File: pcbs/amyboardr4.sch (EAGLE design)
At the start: 129 parts, among them J1 52601-G10-8LF, M13 M2.5, M14 M2.5, M15 M2.5, M16 M2.5, Q2 S8050, Q5 S8050, U1 PCM9211PT, U13 HX3608, U15 H11L1SR2M, U16 SPX3819, U2 ESP32­S2­SOLO, Y1 ABM10W-22.5792MHZ-8-K1Z-T3

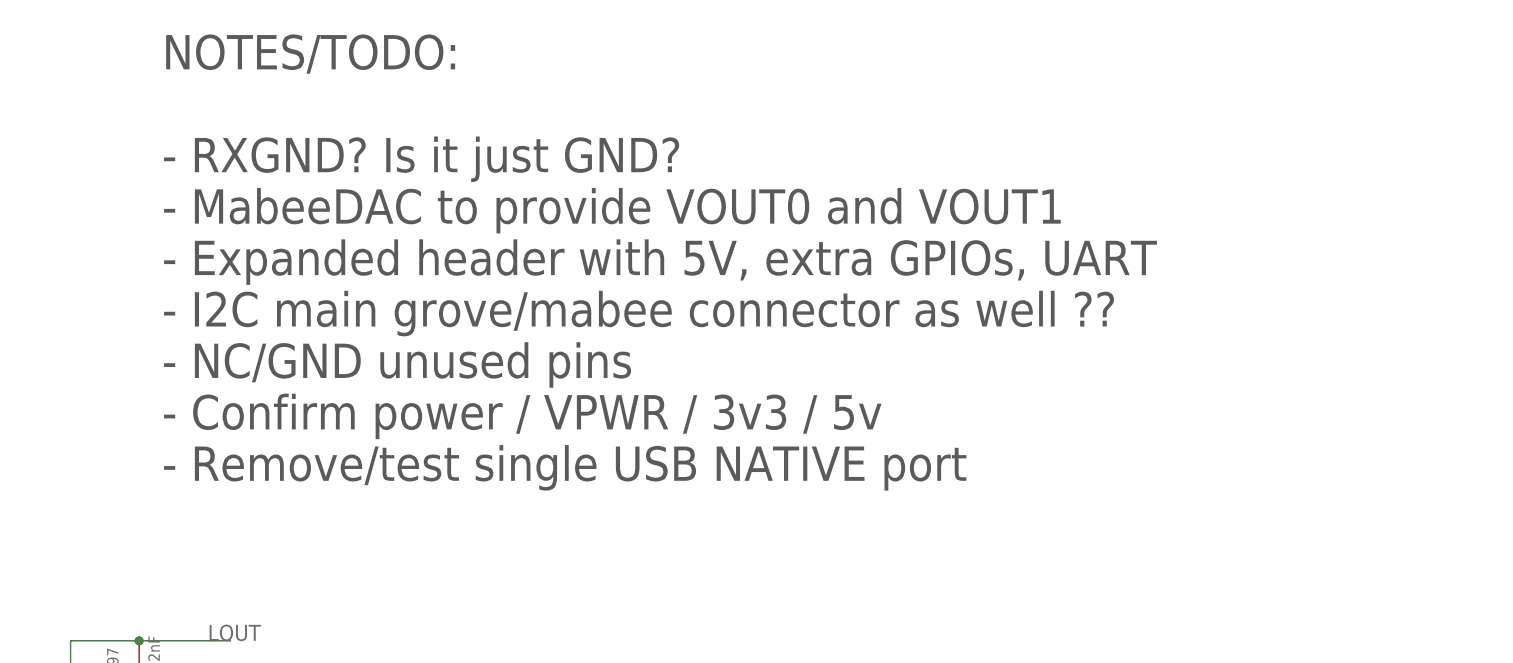
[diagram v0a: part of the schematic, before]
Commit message: .
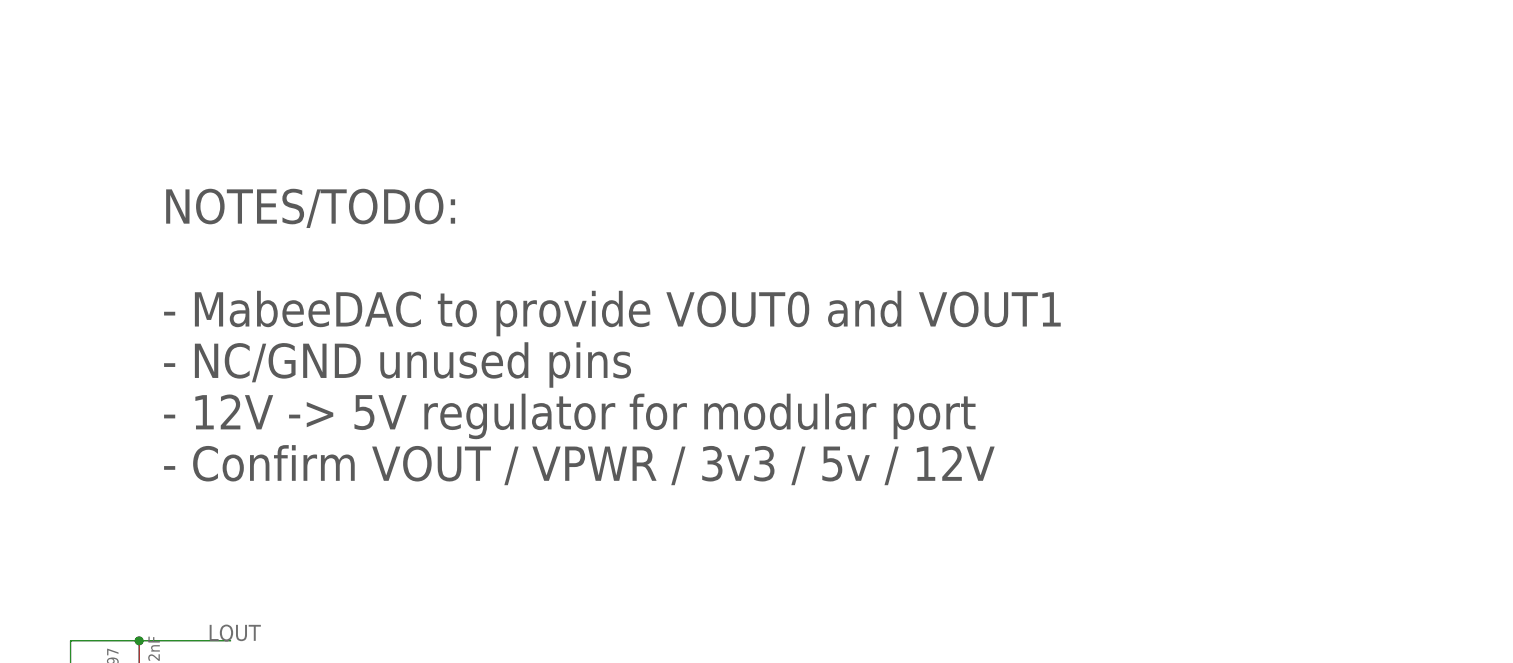
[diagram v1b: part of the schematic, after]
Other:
- note added: "NOTES/TODO: - MabeeDAC to provide VOUT0 and VOUT1 - NC/GND unused pins - 12V -> 5V regulator for modular port - Confirm VOUT / VPWR / 3v3 / 5v / 12V"
- note removed: "NOTES/TODO: - RXGND? Is it just GND? - MabeeDAC to provide VOUT0 and VOUT1 - Expanded header with 5V, extra GPIOs, UART - I2C main grove/mabee connector as well ?? - NC/GND unused pins - Confirm power / VPWR / 3v3 / 5v - Remove/test single USB NATIVE port"
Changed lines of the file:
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@@
 <text x="192.786" y="113.538" size="5.08" layer="97">HEADERS</text>
 <text x="294.64" y="190.5" size="3.81" layer="97">NOTES/TODO:
-- RXGND? Is it just GND?
 - MabeeDAC to provide VOUT0 and VOUT1
-- Expanded header with 5V, extra GPIOs, UART
-- I2C main grove/mabee connector as well ??
 - NC/GND unused pins
-- Confirm power / VPWR / 3v3 / 5v
-- Remove/test single USB NATIVE port</text>
+- 12V -&gt; 5V regulator for modular port
+- Confirm VOUT / VPWR / 3v3 / 5v / 12V
+</text>
 <text x="129.54" y="-54.61" size="5.08" layer="97">TF Card</text>
 <text x="193.548" y="-73.406" size="1.778" layer="97">D3</text>
